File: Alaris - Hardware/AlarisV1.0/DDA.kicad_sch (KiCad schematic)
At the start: 26 parts, among them J3 636101111001, U10 BMP280, U2 BNO055, U4 MS5611-01BA, U5 ICM-20948, U8 NEO-M8N, Y1 32k768

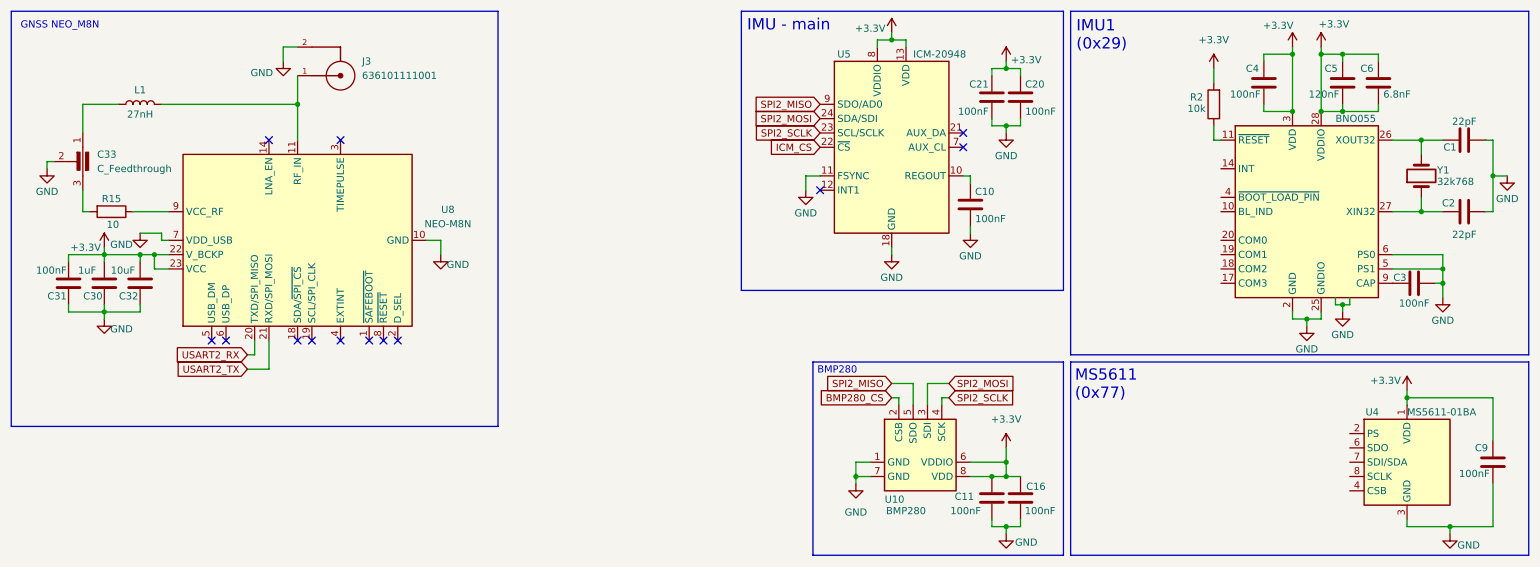
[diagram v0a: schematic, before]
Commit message: Desenvolvimento da PCB
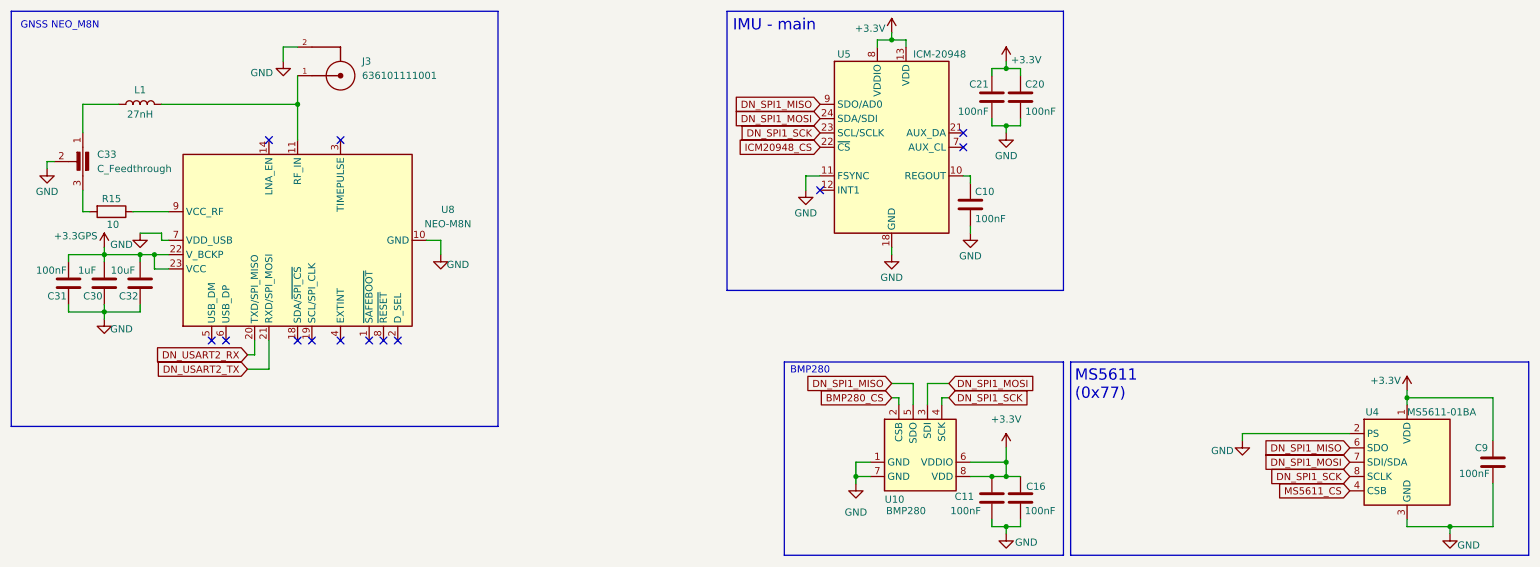
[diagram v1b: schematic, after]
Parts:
- removed C1, C2: 22pF, Capacitor_SMD:C_0603_1608Metric_Pad1.08x0.95mm_HandSolder, symbol Device:C
- removed C3, C4: 100nF, Capacitor_SMD:C_0603_1608Metric_Pad1.08x0.95mm_HandSolder, symbol Device:C
- removed C5: 120nF, Capacitor_SMD:C_0603_1608Metric_Pad1.08x0.95mm_HandSolder, symbol Device:C
- removed C6: 6.8nF, Capacitor_SMD:C_0603_1608Metric_Pad1.08x0.95mm_HandSolder, symbol Device:C
- removed R2: 10k, Resistor_SMD:R_0603_1608Metric_Pad0.98x0.95mm_HandSolder, symbol Device:R
- removed U2: BNO055, Package_LGA:LGA-28_5.2x3.8mm_P0.5mm, symbol Sensor_Motion:BNO055
- removed Y1: 32k768, Crystal:Crystal_SMD_0603-4Pin_6.0x3.5mm_HandSoldering, symbol Device:Crystal
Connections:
- net SPI2_MISO is gone; now on net DN_SPI1_MISO: U10.5 (SDO), U5.9 (SDO/AD0)
- net SPI2_MOSI is gone; now on net DN_SPI1_MOSI: U10.3 (SDI), U5.24 (SDA/SDI)
- net SPI2_SCLK is gone; now on net DN_SPI1_SCK: U10.4 (SCK), U5.23 (SCL/SCLK)
- net +3.3V: no longer C30.2, C31.2, C32.2, U8.22 (V_BCKP), U8.23 (VCC)
- net GND: now also U4.2 (PS)
- net MS5611_CS: now reaches U4.4 (CSB), U4.5 (CSB)
- net DN_SPI1_MISO: now reaches U4.6 (SDO)
- net DN_SPI1_MOSI: now reaches U4.7 (SDI/SDA)
- net DN_SPI1_SCK: now reaches U4.8 (SCLK)
- net ICM_CS renamed ICM20948_CS
- net USART2_RX renamed DN_USART2_RX
- net USART2_TX renamed DN_USART2_TX
- new net +3.3GPS: C30.2, C31.2, C32.2, U8.22 (V_BCKP), U8.23 (VCC)
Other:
- note removed: "IMU1 (0x29)"
